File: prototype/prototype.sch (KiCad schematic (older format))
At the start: 33 parts, among them P1 CONN_25X2, P2 CONN_25X2, P3 VGACONN, U1 MC68SEC000

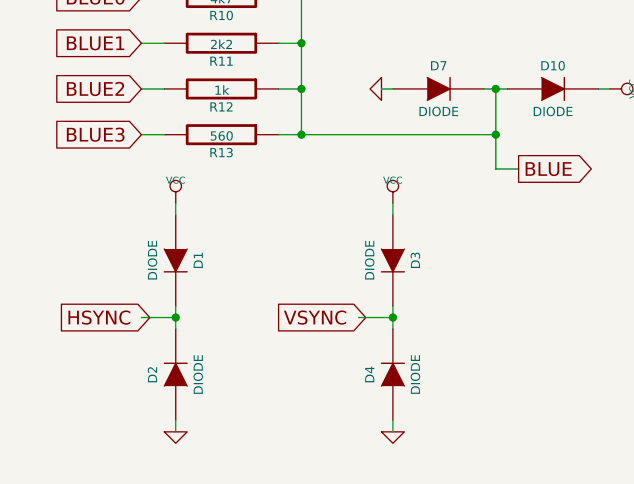
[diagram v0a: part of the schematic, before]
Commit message: PCB floor planning.
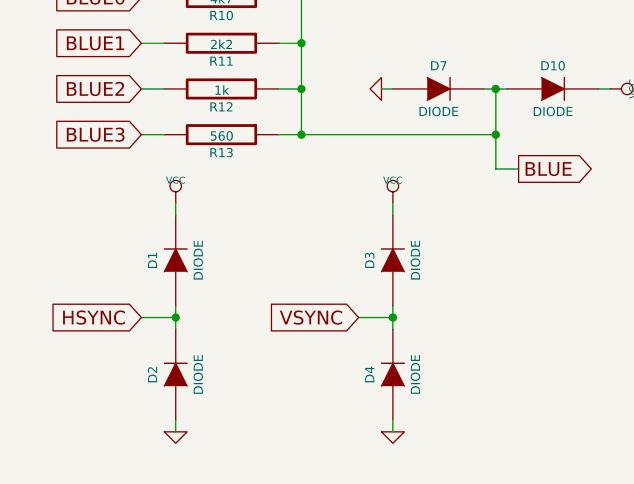
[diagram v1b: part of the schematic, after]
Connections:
- net HSYNC: now also D1.1 (A), D2.2 (K)
- net VCC: now also D1.2 (K), D3.2 (K); no longer D1.1 (A), D3.1 (A)
- net VSYNC: now also D3.1 (A), D4.2 (K)
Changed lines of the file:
@@
 	2650 4500 2750 4500
 Connection ~ 2650 4350
-Text GLabel 750  7150 2    60   Output ~ 0
+Text GLabel 1100 7150 0    60   Input ~ 0
 HSYNC
 $Comp
@@
 F 3 "" H 1250 6900 60  0000 C CNN
 	1    1250 6900
-	0    1    1    0
+	0    -1   -1   0
 $EndComp
 Wire Wire Line
 	1250 7100 1250 7200
-Wire Wire Line
-	1100 7150 1250 7150
 Connection ~ 1250 7150
 $Comp
@@
 Wire Wire Line
 	1250 7600 1250 7650
-Text GLabel 1700 7150 2    60   Output ~ 0
+Text GLabel 2050 7150 0    60   Input ~ 0
 VSYNC
 $Comp
@@
 F 3 "" H 2200 6900 60  0000 C CNN
 	1    2200 6900
-	0    1    1    0
+	0    -1   -1   0
 $EndComp
 Wire Wire Line
 	2200 7100 2200 7200
-Wire Wire Line
-	2050 7150 2200 7150
 Connection ~ 2200 7150
 $Comp
@@
 Wire Wire Line
 	3350 1500 3400 1500
+Wire Wire Line
+	2050 7150 2200 7150
+Wire Wire Line
+	1100 7150 1250 7150
 $EndSCHEMATC
